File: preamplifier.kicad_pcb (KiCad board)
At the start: 2 copper layers, 81.3 x 58.4 mm, 63 parts, among them SW1L1 SW_DIP_x04, SW1R1 SW_DIP_x04, U1 OPA2134, U2 OPA2134

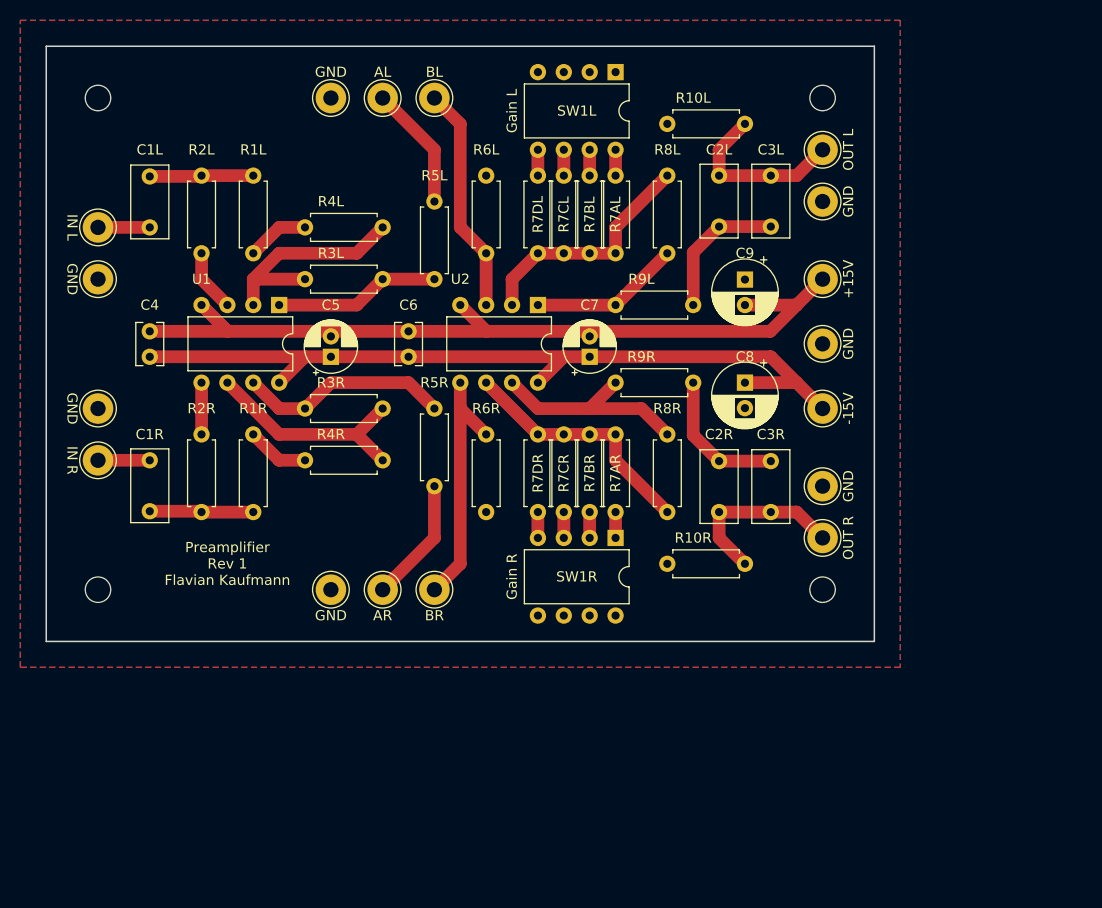
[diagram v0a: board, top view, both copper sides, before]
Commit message: cosmetics
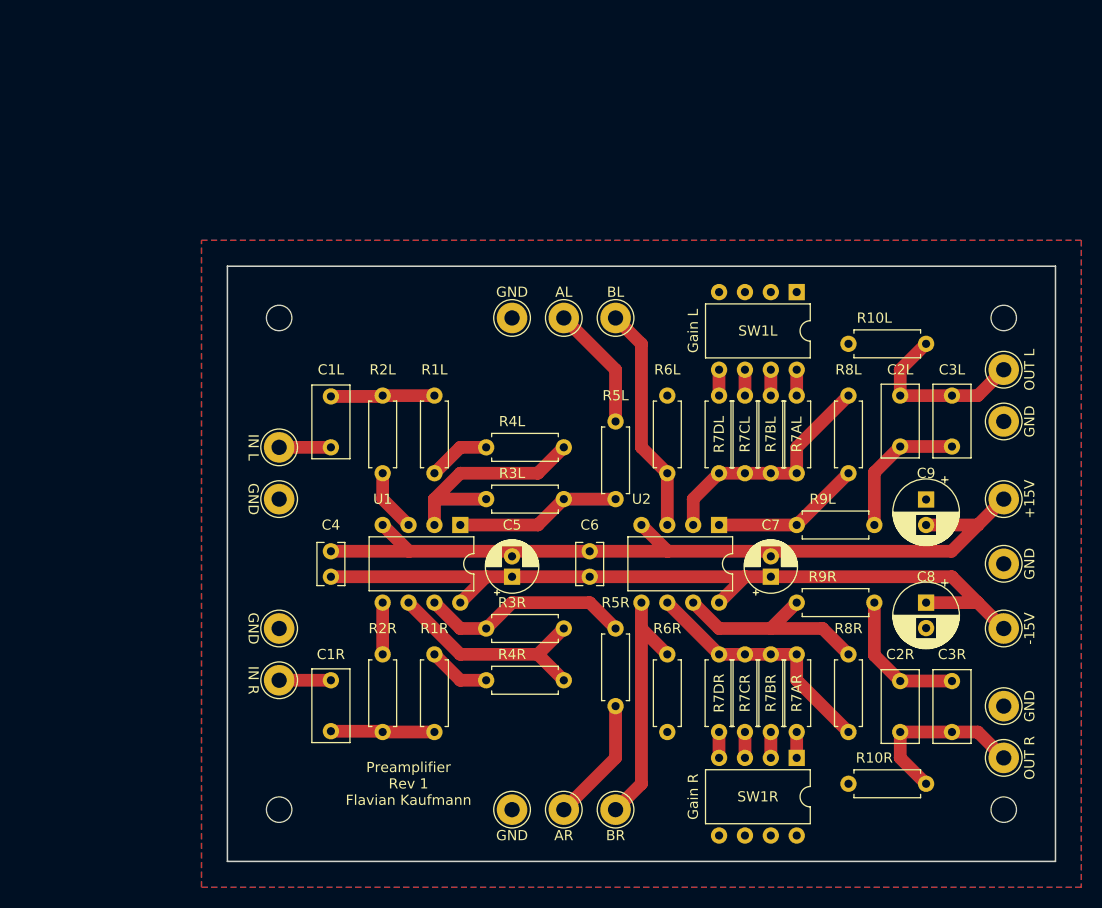
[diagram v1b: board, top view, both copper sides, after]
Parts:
- moved R3R1 28.0 mm to (132.1, 102.9)
- moved R6R1 28.0 mm to (142.2, 105.4)
- moved REF** 28.0 mm to (132.1, 72.4)
- moved REF** 28.0 mm to (132.1, 120.7)
- moved C1L1 28.0 mm to (109.2, 85.1)
- moved C1R1 28.0 mm to (109.2, 108.0)
- moved C2L1 28.0 mm to (165.1, 85.0)
- moved C2L2 28.0 mm to (165.1, 108.0)
- moved C3L1 28.0 mm to (170.2, 80.0)
- moved C3L2 28.0 mm to (170.2, 113.0)
- moved C4 28.0 mm to (109.2, 97.8)
- moved C5 28.0 mm to (127.0, 97.8)
- moved C6 28.0 mm to (134.6, 97.8)
- moved C7 28.0 mm to (152.4, 97.8)
- moved R1L1 28.0 mm to (119.4, 80.0)
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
